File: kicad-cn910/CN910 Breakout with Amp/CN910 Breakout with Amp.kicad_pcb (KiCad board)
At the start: 2 copper layers, 45.8 x 32.5 mm, 33 parts, among them J1 CN910_FPC_CON, J2 PB_RF_OUT, J3 USB4125-GF-A-0190_REVA2, SW1 SW_SPDT, U1 ADA4857, U2 AP7375-50SR-7

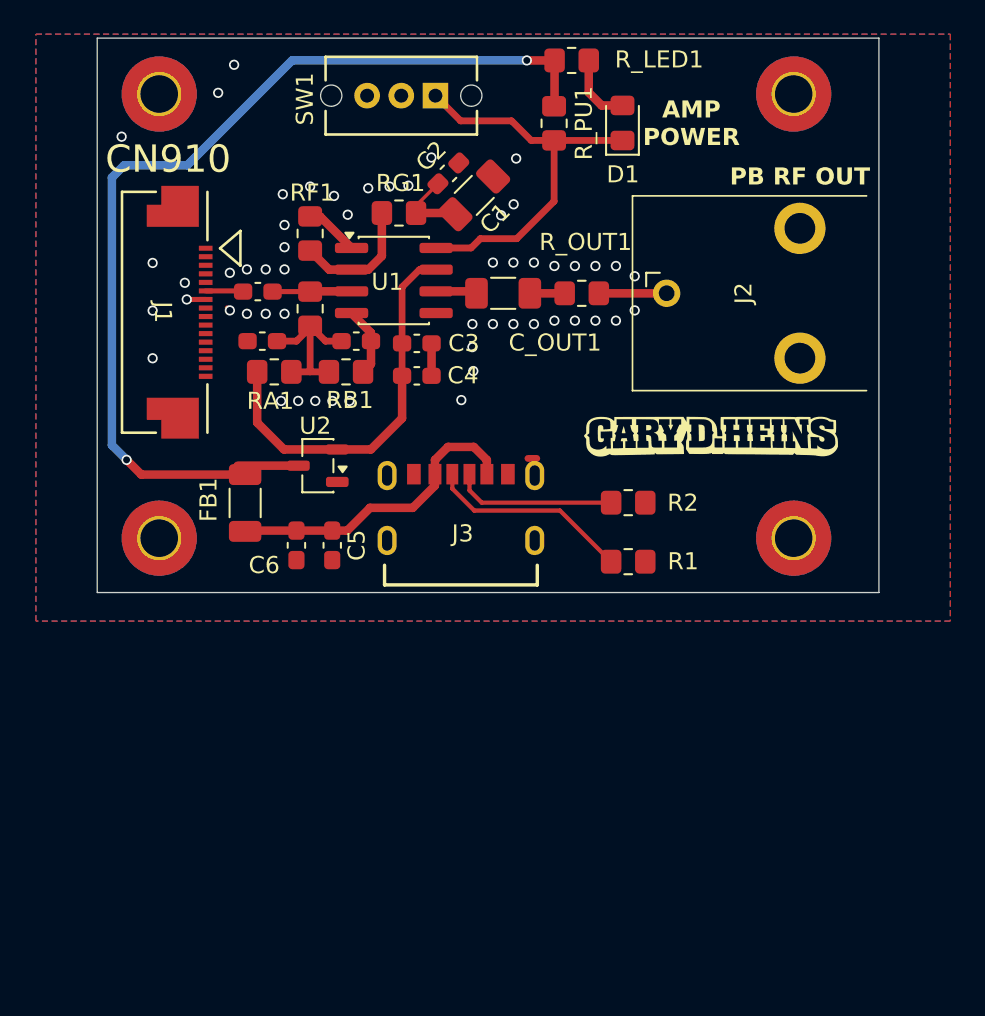
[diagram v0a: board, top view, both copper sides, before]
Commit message: Refactor code structure for improved readability and maintainability
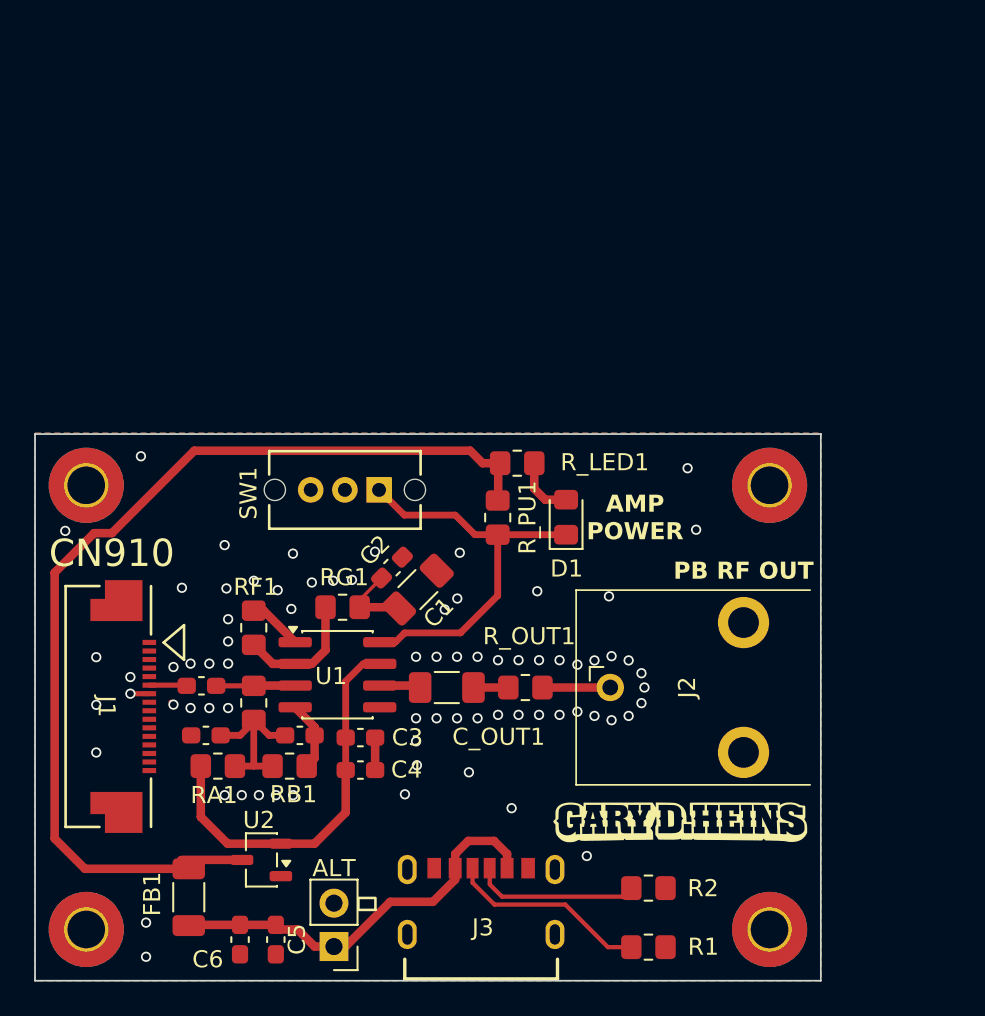
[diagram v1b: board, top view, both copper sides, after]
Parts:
- added REF**: PinHeader_1x02_P2.54mm_Vertical, Connector_PinHeader_2.54mm:PinHeader_1x02_P2.54mm_Vertical, F.Cu at (117.5, 130.0)
- added SONY_AMP**: Board, PCM_kikit:Board, F.Cu at (100.0, 100.0)
- moved R_LED1 23.8 mm to (128.2, 101.7)
- moved C3 23.3 mm to (119.0, 117.8)
- moved C_IN1 23.3 mm to (109.7, 114.7)
- moved D1 23.3 mm to (131.1, 104.9)
- moved FB1 23.3 mm to (109.0, 127.1)
- moved J2 23.3 mm to (133.7, 114.8)
- moved RB1 23.3 mm to (114.9, 119.4)
- moved R_BIAS1 23.3 mm to (112.8, 115.7)
- moved U2 23.3 mm to (113.3, 124.9)
- moved C_VREF_A1 23.3 mm to (110.0, 117.6)
- moved RG1 23.3 mm to (118.0, 110.1)
- moved C1 23.3 mm to (122.4, 109.1)
- moved C2 23.3 mm to (120.9, 107.8)
- moved C4 23.3 mm to (119.0, 119.7)
- moved C5 23.3 mm to (114.1, 129.6)
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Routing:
- net /USB Power/USB_5V: track 18.5 -> 24.0 mm
- net Net-(D1-A): track 4.17 -> 3.62 mm
- net GND: track 7.85 -> 7.33 mm, vias 54 -> 75
- net /Amplifier/USB_5V: track 59.1 -> 59.2 mm, vias 2 -> 0
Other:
- board size 45.8 x 32.5 mm -> 46 x 32 mm
- board text added: "5.2-45V"
- board text added: "ALT"
- board text added: "⏚"
